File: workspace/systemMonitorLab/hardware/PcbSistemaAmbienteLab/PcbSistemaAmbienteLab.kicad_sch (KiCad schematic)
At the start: 2 parts

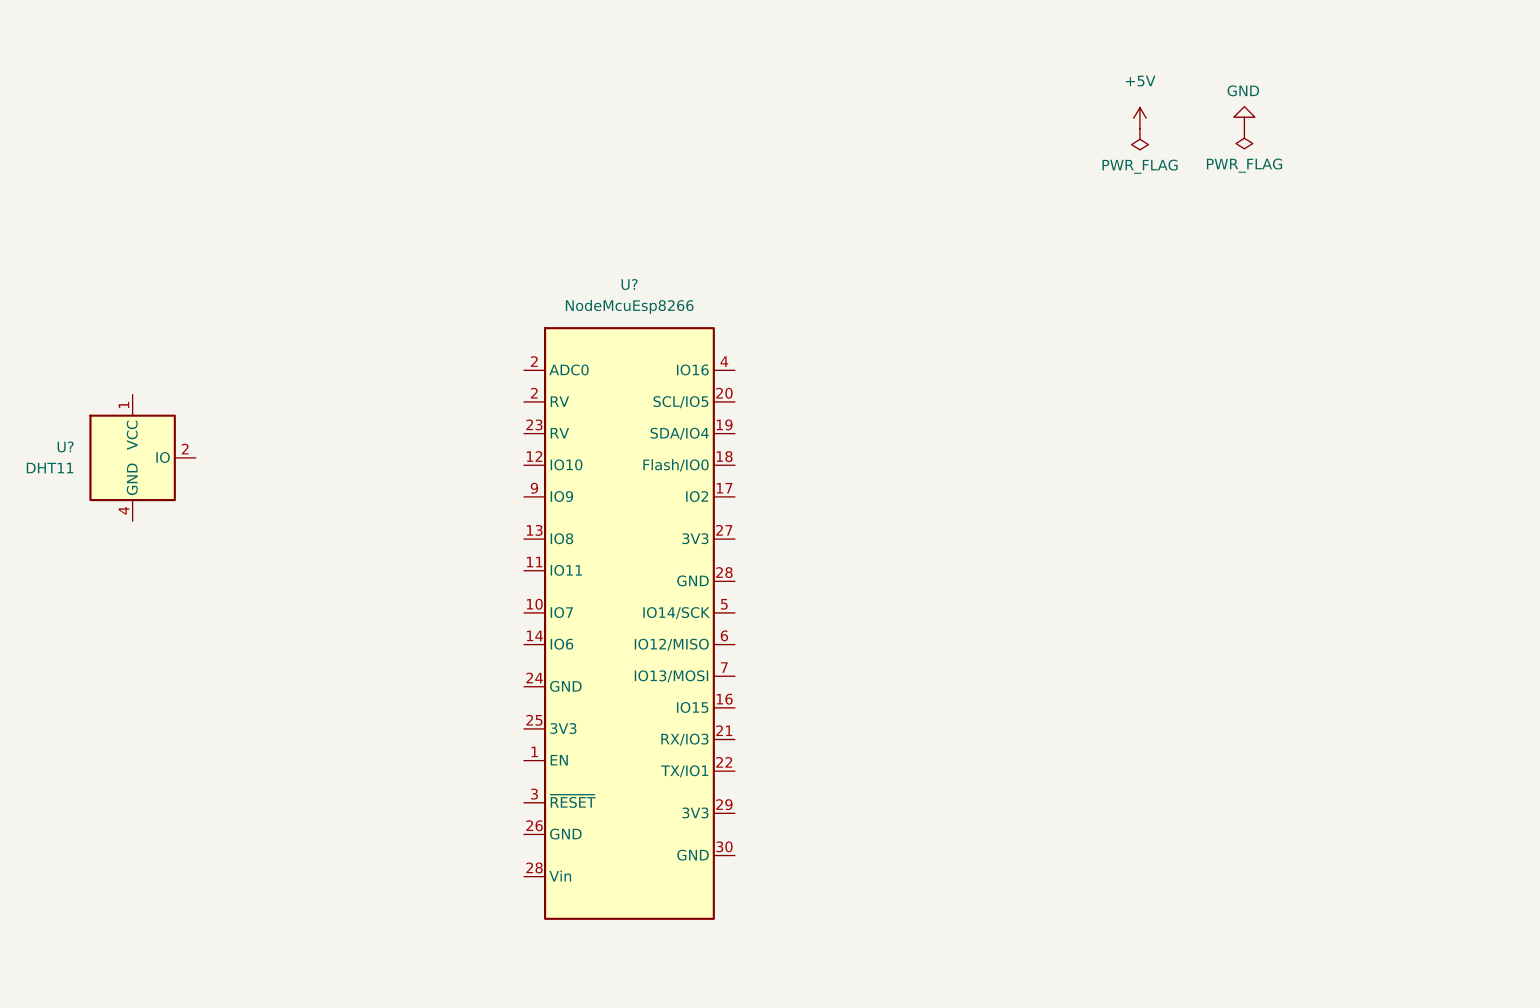
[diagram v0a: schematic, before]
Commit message: Esquemativo v1.0 y PCB v1.0
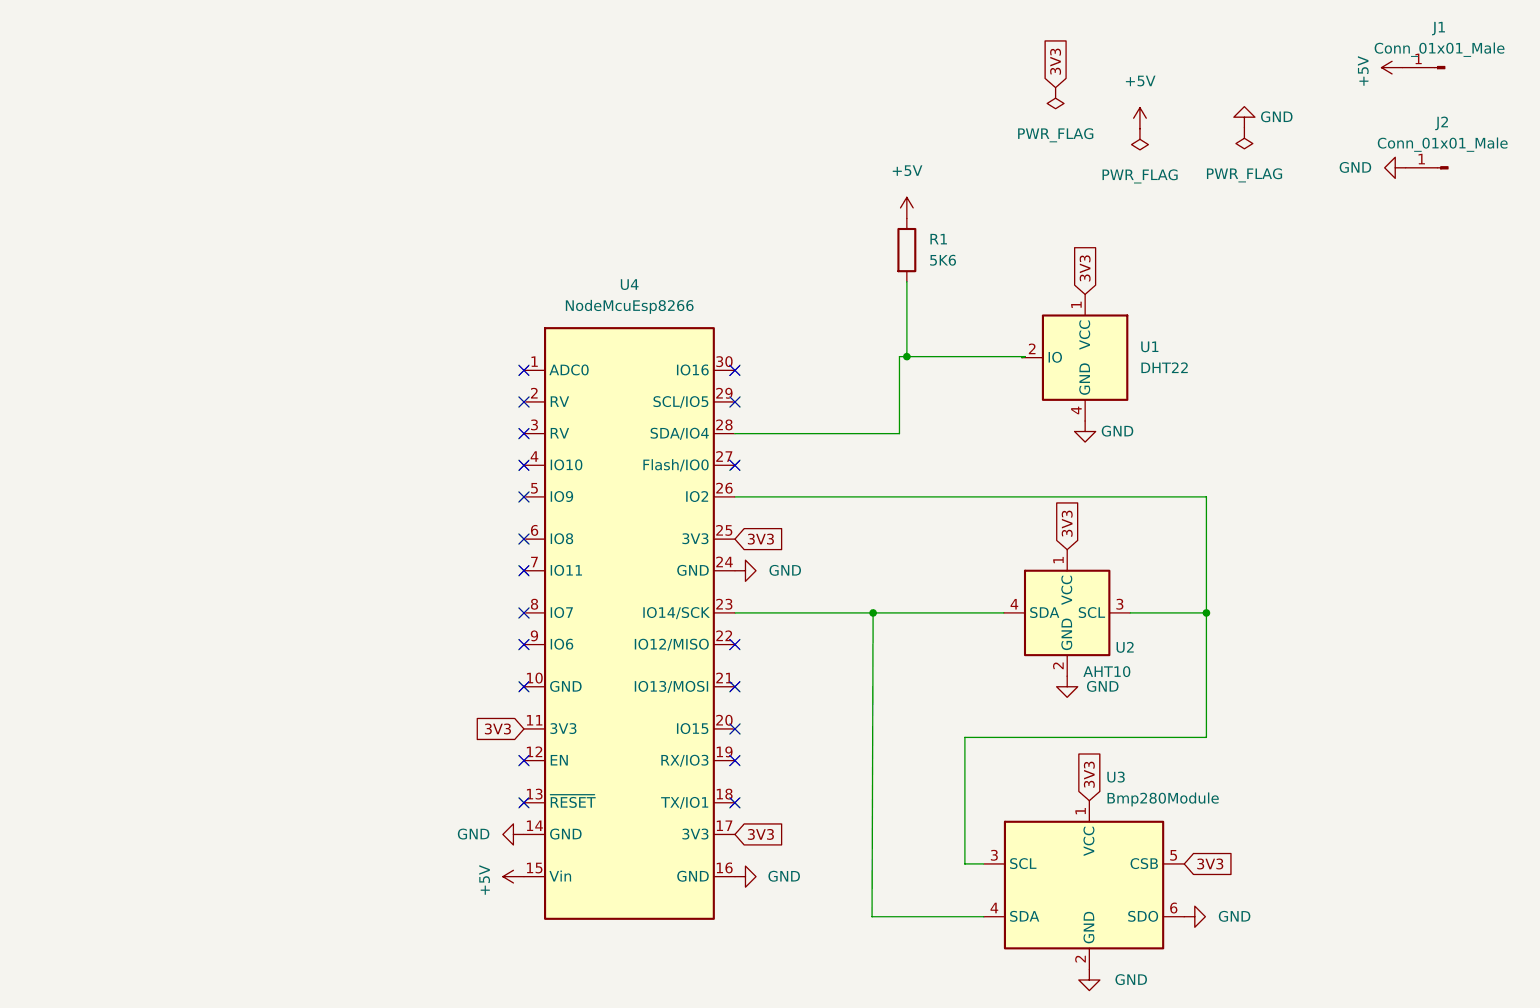
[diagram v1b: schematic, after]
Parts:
- removed U?: DHT11, Sensor:Aosong_DHT11_5.5x12.0_P2.54mm, symbol Sensor:DHT11
- added J1, J2: Conn_01x01_Male, Connector_Pin:Pin_D1.0mm_L10.0mm, symbol Connector:Conn_01x01_Male
- added R1: 5K6, Resistor_THT:R_Axial_DIN0411_L9.9mm_D3.6mm_P12.70mm_Horizontal, symbol Device:R
- added U1: DHT22, Sensor:Aosong_DHT11_5.5x12.0_P2.54mm, symbol New_Library:DHT22
- added U2: AHT10, Connector_PinHeader_2.54mm:PinHeader_1x04_P2.54mm_Vertical, symbol New_Library:AHT10
- added U3: Bmp280Module, Connector_PinHeader_2.54mm:PinHeader_1x06_P2.54mm_Vertical, symbol New_Library:Bmp280Module
- U4: renamed from U?; footprint Module:Adafruit_Feather_32u4_FONA -> NodeMCU_Module:ES8266
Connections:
- net +5V: now also U4.15 (Vin), J1.1 (Pin_1), R1.1
- net GND: now also U4.14 (GND), U4.16 (GND), U4.24 (GND), J2.1 (Pin_1), U1.4 (GND), U2.2 (GND), U3.2 (GND), U3.6 (SDO)
- net 3V3: now reaches U4.11 (3V3)
- net 3V3: now also U4.17 (3V3), U4.25 (3V3), U1.1 (VCC), U2.1 (VCC), U3.1 (VCC), U3.5 (CSB)
- net at U4.23 (IO14/SCK): now also U2.4 (SDA), U3.4 (SDA)
- net at U4.26 (IO2): now also U2.3 (SCL), U3.3 (SCL)
- net at U4.28 (SDA/IO4): now also R1.2, U1.2 (IO)
- no-connect marks 0 -> 20
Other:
- company: (none) -> Servicio Meteorológico Nacional (SMN)
- title: (none) -> Sensores de temperatura, humedad y presión
